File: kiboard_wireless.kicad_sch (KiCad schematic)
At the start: 117 parts, among them J1 USB_C_Receptacle_USB2.0_16P, J2 Conn_01x02_Shielded, J3 TC2030_SWD, Q1 2N7002, SW1 SW_Nidec_CAS-120A1, SW2 SW_Push_45deg, U1 nRF52840_E73-2G4M08S1C, U3 BQ24075RGT, U4 MAX17048, U5 SRV05-4

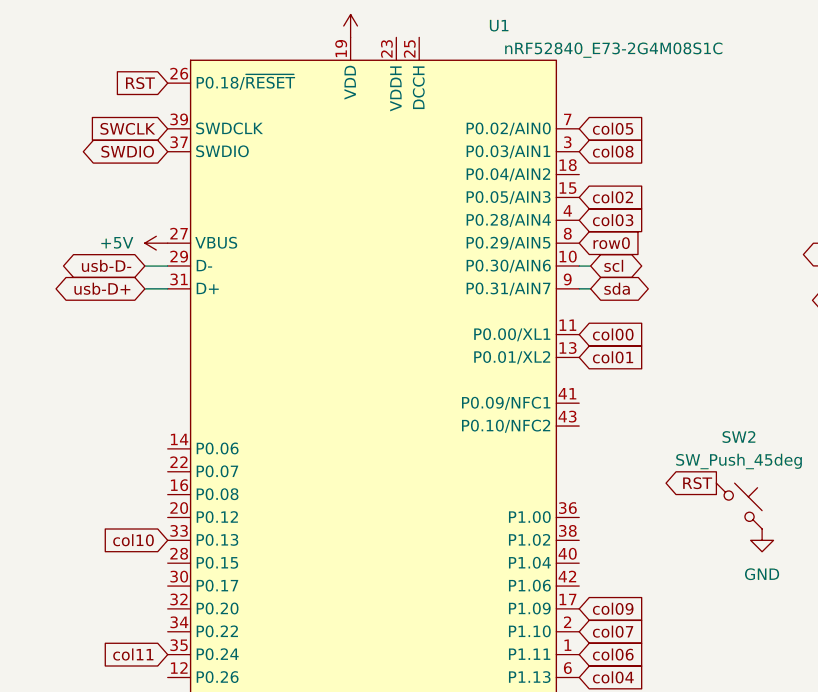
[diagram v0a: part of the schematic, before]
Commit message: improvements
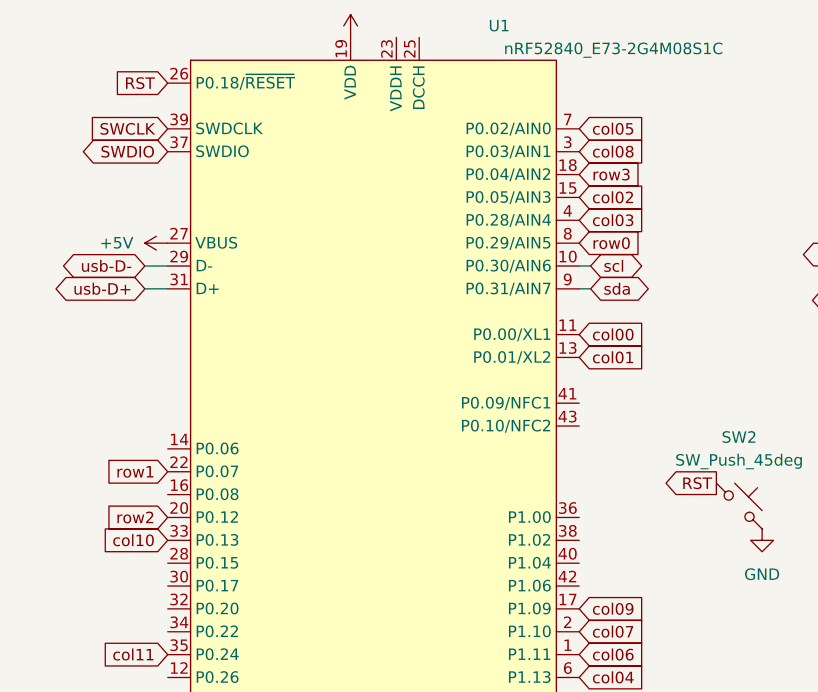
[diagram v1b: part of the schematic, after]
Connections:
- net row1: now also U1.22 (P0.07)
- net row2: now also U1.20 (P0.12)
- net row3: now also U1.18 (P0.04/AIN2)
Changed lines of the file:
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@@
+    )
+  )
+  (global_label "row1" (shape input) (at 39.37 81.28 180) (fields_autoplaced)
+    (effects (font (size 1.27 1.27)) (justify right))
+    (property "Intersheetrefs" "${INTERSHEET_REFS}" (at 31.9096 81.28 0)
+      (effects (font (size 1.27 1.27)) (justify right) hide)
     )
   )
@@
     )
   )
+  (global_label "row3" (shape input) (at 85.09 48.26 0) (fields_autoplaced)
+    (effects (font (size 1.27 1.27)) (justify left))
+    (property "Intersheetrefs" "${INTERSHEET_REFS}" (at 92.5504 48.26 0)
+      (effects (font (size 1.27 1.27)) (justify left) hide)
+    )
+  )
   (global_label "col10" (shape input) (at 39.37 88.9 180) (fields_autoplaced)
     (effects (font (size 1.27 1.27)) (justify right))
@@
     )
   )
+  (global_label "row2" (shape input) (at 39.37 86.36 180) (fields_autoplaced)
+    (effects (font (size 1.27 1.27)) (justify right))
+    (property "Intersheetrefs" "${INTERSHEET_REFS}" (at 31.9096 86.36 0)
+      (effects (font (size 1.27 1.27)) (justify right) hide)
+    )
+  )

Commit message: cosmetic improvements
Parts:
- J3: footprint PCM_marbastlib-various:CON_TC2030_outlined -> paw:Paw-Connect_RevB_TC2030-IDC-NL_2x03_P1.27mm_Vertical
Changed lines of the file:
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@@
       (effects (font (size 1.27 1.27)) (justify left))
     )
-    (property "Footprint" "PCM_marbastlib-various:CON_TC2030_outlined" (at 135.89 60.96 90)
+    (property "Footprint" "paw:Paw-Connect_RevB_TC2030-IDC-NL_2x03_P1.27mm_Vertical" (at 135.89 60.96 90)
       (effects (font (size 1.27 1.27)) hide)
     )
